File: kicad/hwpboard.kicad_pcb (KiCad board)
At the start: 2 copper layers, 100 x 80 mm, 24 parts, among them J1 Barrel_Jack_Switch, J2 Conn_01x01, J3 Conn_01x01, J4 Conn_01x01, J5 Conn_01x01, U1 AD8603

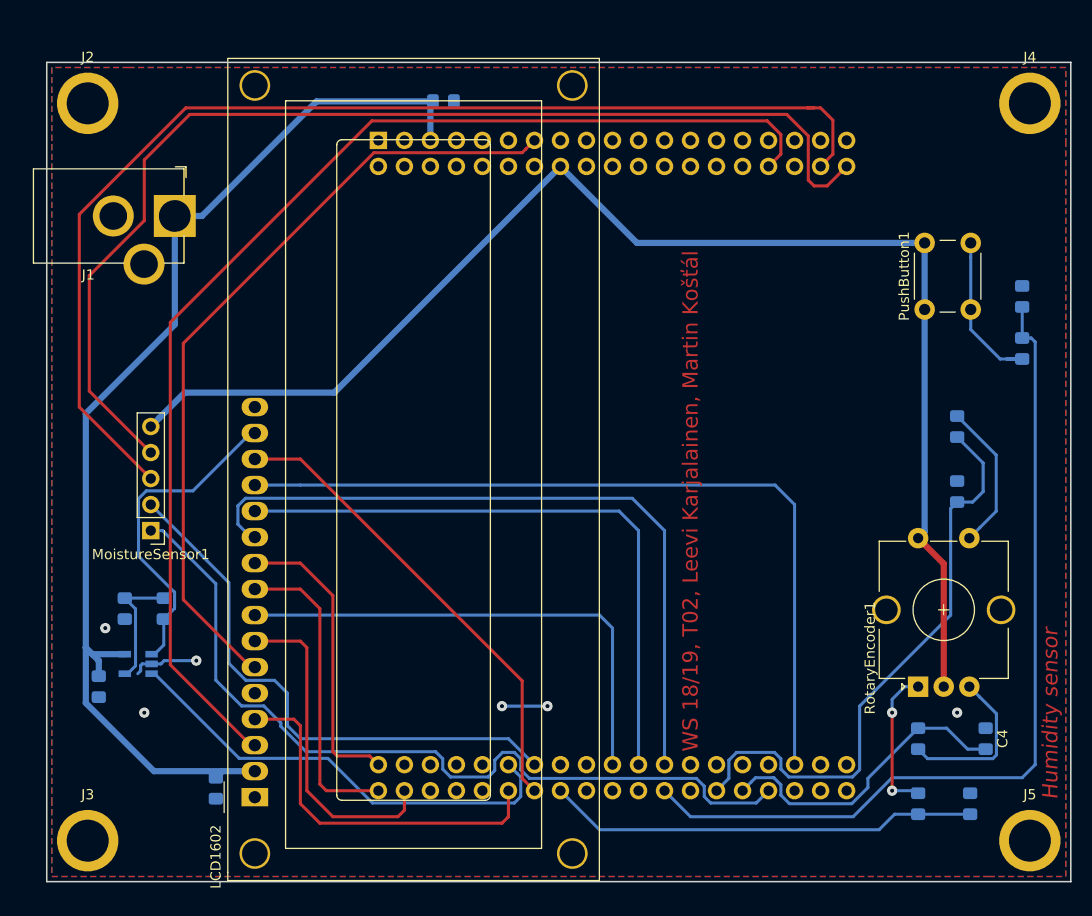
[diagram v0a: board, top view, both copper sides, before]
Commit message: layout_all_routed_and_drc_ok_beta_2.0
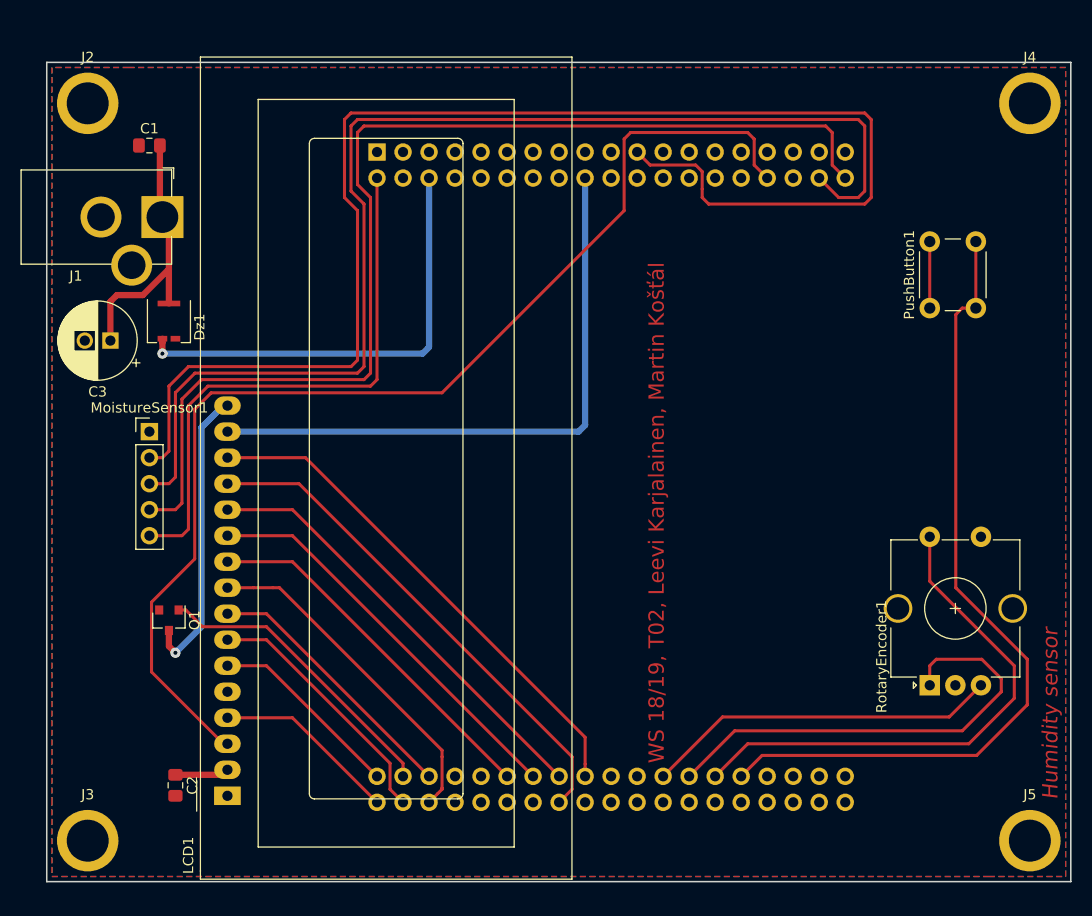
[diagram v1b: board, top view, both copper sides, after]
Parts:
- removed C4, C5, C6, C7: 100n, Capacitor_SMD:C_0805_2012Metric_Pad1.15x1.40mm_HandSolder
- removed LCD1602: RC1602A, HWP:WC1602A
- removed R1: 10k, Resistor_SMD:R_0805_2012Metric_Pad1.15x1.40mm_HandSolder
- removed R2: 6.2k, Resistor_SMD:R_0805_2012Metric_Pad1.15x1.40mm_HandSolder
- removed R3, R4, R5, R6: 50k, Resistor_SMD:R_0805_2012Metric_Pad1.15x1.40mm_HandSolder
- removed U1: AD8603, Package_TO_SOT_SMD:TSOT-23-5
- added Dz1: ZEN056V115A24LS, Diode_SMD:Littelfuse_PolyZen-LS, F.Cu at (120.7, 67.4)
- added LCD1: RC1602A, HWP:WC1602A_no_mount, F.Cu at (126.5, 113.8)
- added Q1: BSS138, Package_TO_SOT_SMD:SOT-23, F.Cu at (120.7, 96.6)
- C1, C2: footprint Capacitor_SMD:C_0805_2012Metric_Pad1.15x1.40mm_HandSolder -> HWP:C_0805_2012Metric_Pad1.15x1.40mm_HandSolder; moved to F.Cu
- C3: value 100n -> 100u; footprint Capacitor_SMD:C_0805_2012Metric_Pad1.15x1.40mm_HandSolder -> HWP:CP_Radial_D7.5mm_P2.50mm; moved to F.Cu
- moved C3 95.4 mm to (115.0, 69.3), turned to 180 degrees
- moved C1 86.5 mm to (118.8, 50.3), turned to 0 degrees
- moved C2 81.5 mm to (121.4, 112.7), turned to 270 degrees
- moved MoistureSensor1 9.66 mm to (118.8, 78.2), turned to 0 degrees
- moved J1 1.21 mm to (120.1, 57.2)
- moved NUCBRD1 1.14 mm to (141.1, 50.9)
- moved RotaryEncoder1 1.14 mm to (195.0, 103.0)
- moved PushButton1 0.52 mm to (195.0, 66.1)
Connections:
- C1 pad 1: btn1 -> GND
- C1 pad 2: GND -> Net-(C1-Pad2)
- C2 pad 1: btn0 -> +5V
- C3 pad 1: rotary0 -> Net-(C1-Pad2)
- J1 pad 1: +5V -> Net-(C1-Pad2)
- MoistureSensor1 pad 1: GNDA -> GND
- MoistureSensor1 pad 2: PWM -> PWM_sensor
- MoistureSensor1 pad 5: +3V3 -> Sensor_enable
- NUCBRD1 pad 13: E -> Net-(NUCBRD1-Pad13)
- NUCBRD1 pad 18: Net-(NUCBRD1-Pad18) -> +5V
- NUCBRD1 pad 2: Net-(NUCBRD1-Pad2) -> Sensor_enable
- NUCBRD1 pad 21: Net-(NUCBRD1-Pad21) -> PWM_sensor
- NUCBRD1 pad 39: d3 -> E
- NUCBRD1 pad 40: d2 -> RS
- NUCBRD1 pad 41: Net-(NUCBRD1-Pad41) -> PWM_LCD
- NUCBRD1 pad 43: Net-(NUCBRD1-Pad43) -> d1
- NUCBRD1 pad 44: Net-(NUCBRD1-Pad44) -> d2
- NUCBRD1 pad 49: DAC1 -> d3
- NUCBRD1 pad 5: +5V -> Net-(NUCBRD1-Pad5)
- NUCBRD1 pad 50: RS -> Net-(NUCBRD1-Pad50)
- NUCBRD1 pad 51: PWM -> d4
- NUCBRD1 pad 52: d7 -> Net-(NUCBRD1-Pad52)
- NUCBRD1 pad 53: Net-(NUCBRD1-Pad53) -> d5
- NUCBRD1 pad 54: rotary0 -> d6
- NUCBRD1 pad 55: Net-(NUCBRD1-Pad55) -> d7
- NUCBRD1 pad 57: d1 -> Net-(NUCBRD1-Pad57)
- NUCBRD1 pad 59: d5 -> Net-(NUCBRD1-Pad59)
- NUCBRD1 pad 61: d4 -> rotary1
- NUCBRD1 pad 62: btn1 -> Net-(NUCBRD1-Pad62)
- NUCBRD1 pad 63: Net-(NUCBRD1-Pad63) -> rotary0
- NUCBRD1 pad 65: Net-(NUCBRD1-Pad65) -> btn0
- NUCBRD1 pad 66: btn0 -> Net-(NUCBRD1-Pad66)
- NUCBRD1 pad 67: Net-(NUCBRD1-Pad67) -> btn1
- NUCBRD1 pad 68: rotary1 -> Net-(NUCBRD1-Pad68)
- NUCBRD1 pad 70: GNDA -> GND
- NUCBRD1 pad 71: d6 -> Net-(NUCBRD1-Pad71)
- PushButton1 pad 1: +3V3 -> GND
- PushButton1 pad 2: Net-(PushButton1-Pad2) -> btn1
- RotaryEncoder1 pad A: Net-(R5-Pad1) -> rotary0
- RotaryEncoder1 pad B: Net-(R6-Pad1) -> rotary1
- RotaryEncoder1 pad C: +3V3 -> GND
- RotaryEncoder1 pad S1: +3V3 -> btn0
- RotaryEncoder1 pad S2: Net-(R4-Pad2) -> GND
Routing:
- net PWM_sensor: track 0.00 -> 138.3 mm
- net +3V3: track 133.8 -> 0.00 mm
- net GNDA: track 81.9 -> 0.00 mm
- net E: track 77.2 -> 19.1 mm
- net Sensor_enable: track 0.00 -> 55.3 mm
- net PWM: track 54.5 -> 0.00 mm
- net +5V: track 111.6 -> 64.6 mm
- net DAC1: track 45.1 -> 0.00 mm
- net Net-(Dz1-Pad3): track 0.00 -> 44.3 mm, vias 0 -> 1
- net d4: track 70.1 -> 39.6 mm
- net PWM_LCD: track 0.00 -> 29.4 mm
- net d6: track 78.9 -> 49.7 mm
- net Net-(C1-Pad2): track 0.00 -> 26.6 mm
- net d1: track 48.8 -> 26.3 mm
- net RS: track 36.2 -> 18.0 mm
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
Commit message: Board finished and checked
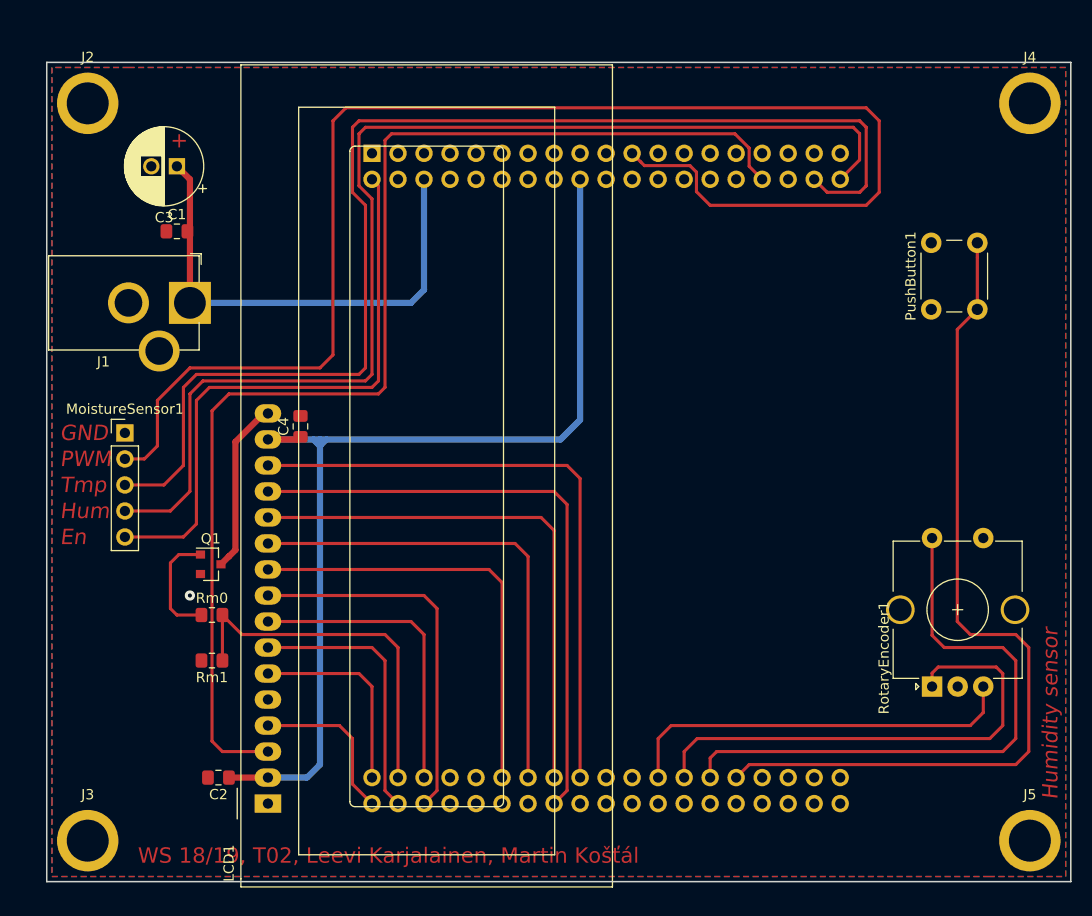
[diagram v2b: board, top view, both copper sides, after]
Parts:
- removed Dz1: ZEN056V115A24LS, Diode_SMD:Littelfuse_PolyZen-LS
- added C4: 100n, HWP:C_0805_2012Metric_Pad1.15x1.40mm_HandSolder, F.Cu at (133.6, 77.7)
- added Rm0: 100, HWP:R_0805_2012Metric_Pad1.15x1.40mm_HandSolder, F.Cu at (124.9, 96.1)
- added Rm1: 10000, HWP:R_0805_2012Metric_Pad1.15x1.40mm_HandSolder, F.Cu at (124.9, 100.5)
- moved C3 18.2 mm to (121.5, 52.3)
- moved C1 8.80 mm to (121.5, 58.6)
- moved J1 8.80 mm to (122.8, 65.6)
- moved Q1 6.82 mm to (124.8, 91.2), turned to 0 degrees
- moved C2 4.27 mm to (125.6, 112.0), turned to 180 degrees
- moved LCD1 4.03 mm to (130.4, 114.5)
- moved MoistureSensor1 2.40 mm to (116.4, 78.3)
- moved NUCBRD1 0.51 mm to (140.6, 51.0)
- moved RotaryEncoder1 0.26 mm to (195.3, 103.1)
- moved PushButton1 0.19 mm to (195.2, 66.3)
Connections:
- J1 pad 3: Net-(J1-Pad3) -> (no net)
- J2 pad 1: Net-(J2-Pad1) -> (no net)
- J3 pad 1: Net-(J3-Pad1) -> (no net)
- J4 pad 1: Net-(J4-Pad1) -> (no net)
- J5 pad 1: Net-(J5-Pad1) -> (no net)
- NUCBRD1 pad 1: Net-(NUCBRD1-Pad1) -> (no net)
- NUCBRD1 pad 10: Net-(NUCBRD1-Pad10) -> (no net)
- NUCBRD1 pad 11: Net-(NUCBRD1-Pad11) -> (no net)
- NUCBRD1 pad 12: Net-(NUCBRD1-Pad12) -> (no net)
- NUCBRD1 pad 13: Net-(NUCBRD1-Pad13) -> (no net)
- NUCBRD1 pad 14: Net-(NUCBRD1-Pad14) -> (no net)
- NUCBRD1 pad 15: Net-(NUCBRD1-Pad15) -> (no net)
- NUCBRD1 pad 16: +3V3 -> (no net)
- NUCBRD1 pad 17: Net-(NUCBRD1-Pad17) -> (no net)
- NUCBRD1 pad 23: Net-(NUCBRD1-Pad23) -> (no net)
- NUCBRD1 pad 24: Net-(NUCBRD1-Pad24) -> (no net)
- NUCBRD1 pad 25: Net-(NUCBRD1-Pad25) -> (no net)
- NUCBRD1 pad 26: Net-(NUCBRD1-Pad26) -> (no net)
- NUCBRD1 pad 27: Net-(NUCBRD1-Pad27) -> (no net)
- NUCBRD1 pad 28: Net-(NUCBRD1-Pad28) -> (no net)
- NUCBRD1 pad 29: Net-(NUCBRD1-Pad29) -> (no net)
- NUCBRD1 pad 3: Net-(NUCBRD1-Pad3) -> (no net)
- NUCBRD1 pad 30: Net-(NUCBRD1-Pad30) -> (no net)
- NUCBRD1 pad 31: Net-(NUCBRD1-Pad31) -> (no net)
- NUCBRD1 pad 33: Net-(NUCBRD1-Pad33) -> (no net)
- NUCBRD1 pad 34: Net-(NUCBRD1-Pad34) -> (no net)
- NUCBRD1 pad 35: Net-(NUCBRD1-Pad35) -> (no net)
- NUCBRD1 pad 37: Net-(NUCBRD1-Pad37) -> (no net)
- NUCBRD1 pad 4: Net-(NUCBRD1-Pad4) -> (no net)
- NUCBRD1 pad 45: Net-(NUCBRD1-Pad45) -> (no net)
- NUCBRD1 pad 46: Net-(NUCBRD1-Pad46) -> (no net)
- NUCBRD1 pad 48: Net-(NUCBRD1-Pad48) -> (no net)
- NUCBRD1 pad 5: Net-(NUCBRD1-Pad5) -> (no net)
- NUCBRD1 pad 50: Net-(NUCBRD1-Pad50) -> (no net)
- NUCBRD1 pad 52: Net-(NUCBRD1-Pad52) -> (no net)
- NUCBRD1 pad 56: Net-(NUCBRD1-Pad56) -> (no net)
- NUCBRD1 pad 57: Net-(NUCBRD1-Pad57) -> (no net)
- NUCBRD1 pad 59: Net-(NUCBRD1-Pad59) -> (no net)
- NUCBRD1 pad 6: Net-(Dz1-Pad3) -> Net-(C1-Pad2)
- NUCBRD1 pad 60: Net-(NUCBRD1-Pad60) -> (no net)
- NUCBRD1 pad 62: Net-(NUCBRD1-Pad62) -> (no net)
- NUCBRD1 pad 64: Net-(NUCBRD1-Pad64) -> (no net)
- NUCBRD1 pad 66: Net-(NUCBRD1-Pad66) -> (no net)
- NUCBRD1 pad 68: Net-(NUCBRD1-Pad68) -> (no net)
- NUCBRD1 pad 69: Net-(NUCBRD1-Pad69) -> (no net)
- NUCBRD1 pad 7: Net-(NUCBRD1-Pad7) -> (no net)
- NUCBRD1 pad 71: Net-(NUCBRD1-Pad71) -> (no net)
- NUCBRD1 pad 72: Net-(NUCBRD1-Pad72) -> (no net)
- NUCBRD1 pad 73: Net-(NUCBRD1-Pad73) -> (no net)
- NUCBRD1 pad 74: Net-(NUCBRD1-Pad74) -> (no net)
- NUCBRD1 pad 75: Net-(NUCBRD1-Pad75) -> (no net)
- NUCBRD1 pad 76: Net-(NUCBRD1-Pad76) -> (no net)
- NUCBRD1 pad 9: Net-(NUCBRD1-Pad9) -> (no net)
- Q1 pad 1: PWM_LCD -> Net-(Q1-Pad1)
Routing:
- net Net-(Dz1-Pad3): track 44.3 -> 0.00 mm, vias 1 -> 0
- net +5V: track 64.6 -> 101.0 mm
- net Net-(C1-Pad2): track 26.6 -> 48.0 mm
- net brightness: track 29.3 -> 16.9 mm, vias 1 -> 0
- net Net-(Q1-Pad1): track 0.00 -> 11.0 mm
- net d7: track 50.0 -> 60.1 mm
- net d6: track 49.7 -> 59.5 mm
- net d5: track 43.2 -> 52.6 mm
- net d4: track 39.6 -> 47.5 mm
- net DAC0: track 112.2 -> 120.1 mm
- net btn0: track 51.6 -> 58.9 mm
- net GND: track 6.50 -> 0.00 mm, vias 0 -> 1
- net d3: track 36.0 -> 42.4 mm
- net PWM_LCD: track 29.4 -> 35.6 mm
- net btn1: track 80.5 -> 85.6 mm
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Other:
- board text added: "+"
- board text added: "-"
- board text added: "En"
- board text added: "GND"
- board text added: "Hum"
- board text added: "PWM"
- board text added: "Tmp"
